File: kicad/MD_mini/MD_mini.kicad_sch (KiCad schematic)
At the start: 46 parts, among them J1 Conn_01x02_Pin, J2 Conn_01x06_Pin, J3 Conn_01x02_Pin, J4 Conn_01x02_Pin, U1 IRS2003, U2 SCM3723ASA, U3 IRS2003, U7 IRS2003, U8 IRS2003, U9 SCM3723ASA

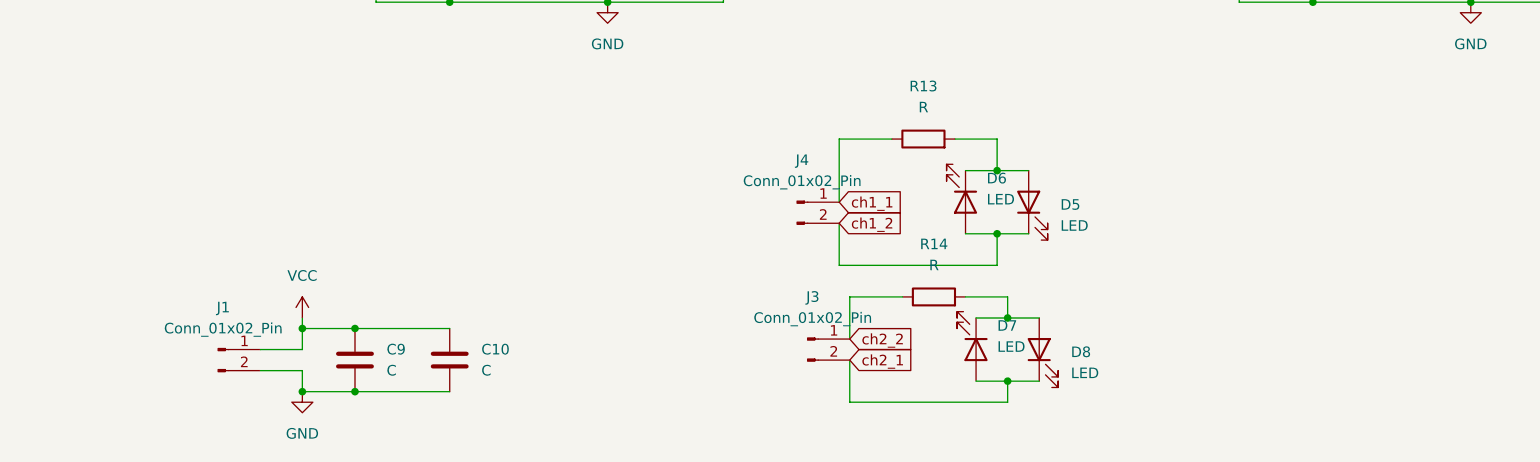
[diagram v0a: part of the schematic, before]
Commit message: a
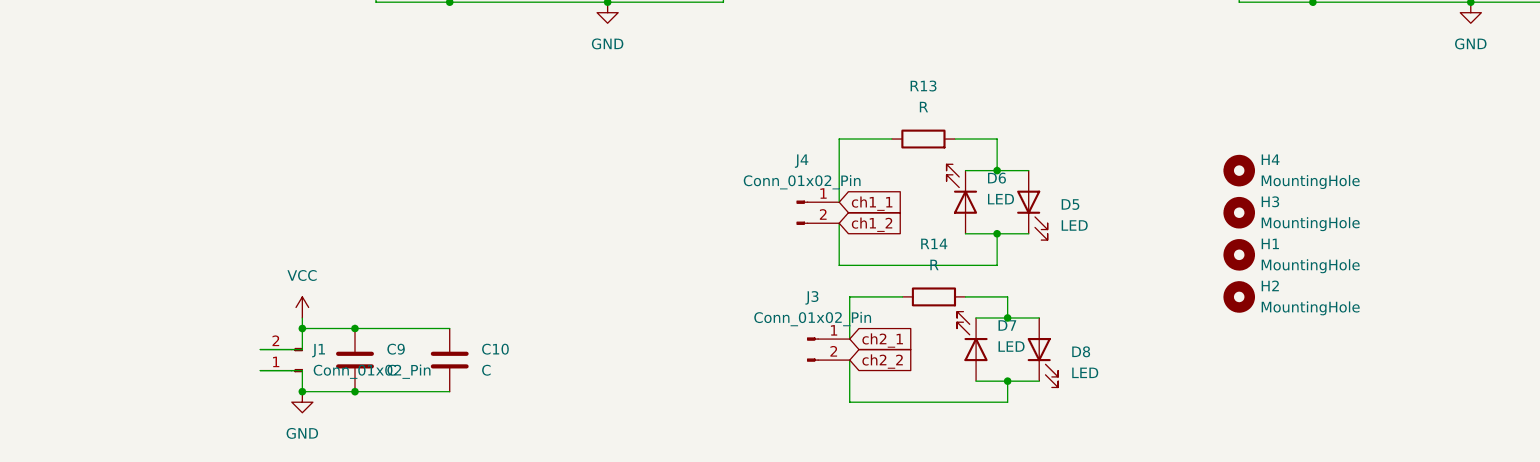
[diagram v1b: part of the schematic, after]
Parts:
- added H1, H2, H3, H4: MountingHole, MountingHole:MountingHole_3.2mm_M3, symbol Mechanical:MountingHole
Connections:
- net GND: now also J1.1 (Pin_1); no longer J1.2 (Pin_2)
- net VCC: now also J1.2 (Pin_2); no longer J1.1 (Pin_1)
- net ch2_1: now also J3.1 (Pin_1), R14.1; no longer D7.2 (A), D8.1 (K), J3.2 (Pin_2)
- net ch2_2: now also D7.2 (A), D8.1 (K), J3.2 (Pin_2); no longer J3.1 (Pin_1), R14.1
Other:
- moved on the sheet: J1

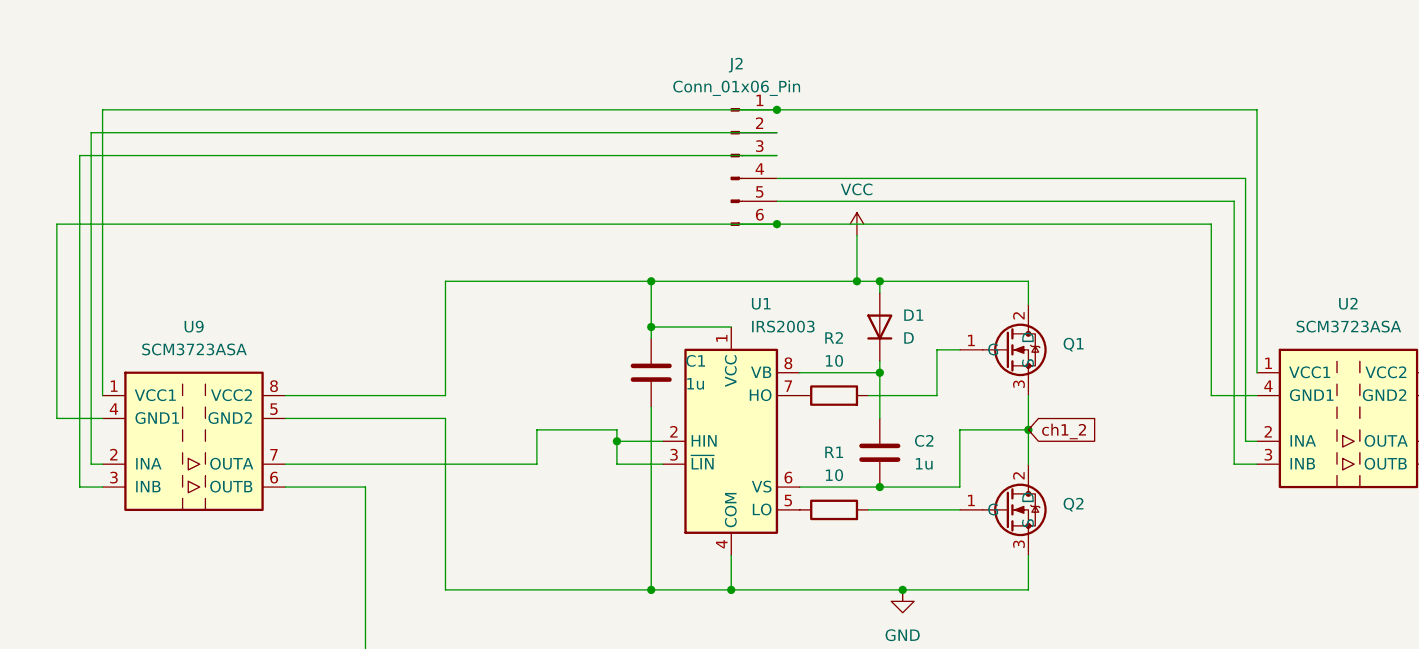
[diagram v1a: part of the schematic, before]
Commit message: a
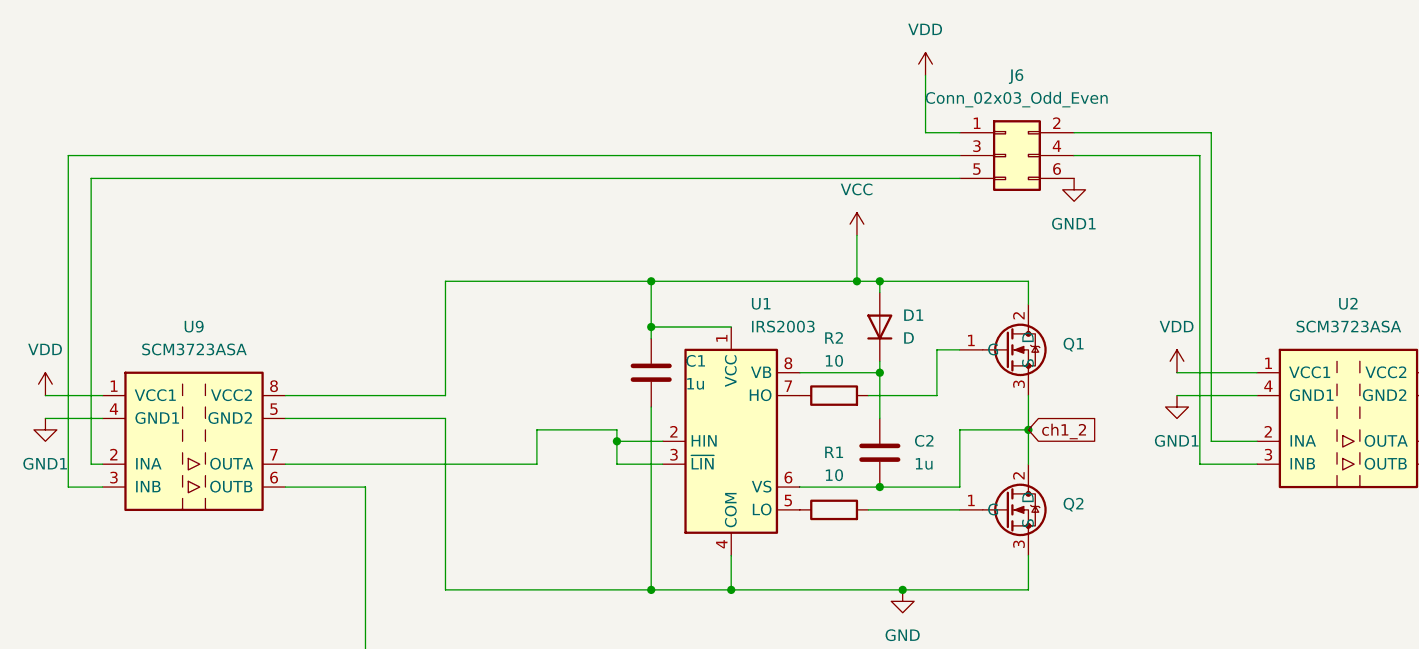
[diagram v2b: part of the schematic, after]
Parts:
- removed J2: Conn_01x06_Pin, Connector_PinHeader_2.54mm:PinHeader_1x06_P2.54mm_Horizontal, symbol Connector:Conn_01x06_Pin
- added J6: Conn_02x03_Odd_Even, Connector_PinHeader_2.54mm:PinHeader_2x03_P2.54mm_Horizontal, symbol Connector_Generic:Conn_02x03_Odd_Even
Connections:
- net VDD: now reaches U2.1 (VCC1), U9.1 (VCC1)
- net VDD: now also J6.1 (Pin_1)
- net at U9.2 (INA): now also J6.5 (Pin_5)
- net at U9.3 (INB): now also J6.3 (Pin_3)
- net GND1: now reaches U2.4 (GND1), U9.4 (GND1)
- net GND1: now also J6.6 (Pin_6)
- net at U2.2 (INA): now also J6.2 (Pin_2)
- net at U2.3 (INB): now also J6.4 (Pin_4)
